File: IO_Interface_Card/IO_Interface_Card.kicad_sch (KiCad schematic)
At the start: 97 parts, among them P1 Conn_02x40_Odd_Even, P2 Conn_02x36_Top_Bottom

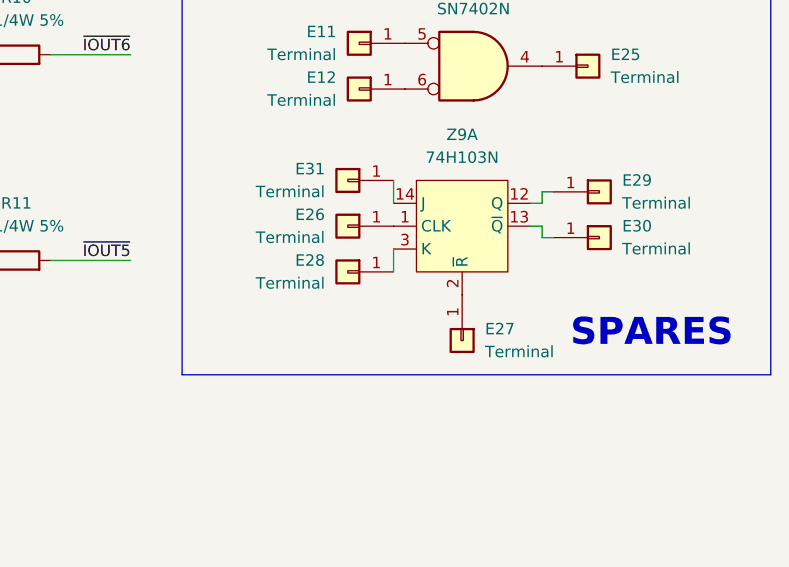
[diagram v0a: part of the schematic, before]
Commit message: Finished Adding Every Chip and Net label in AU1
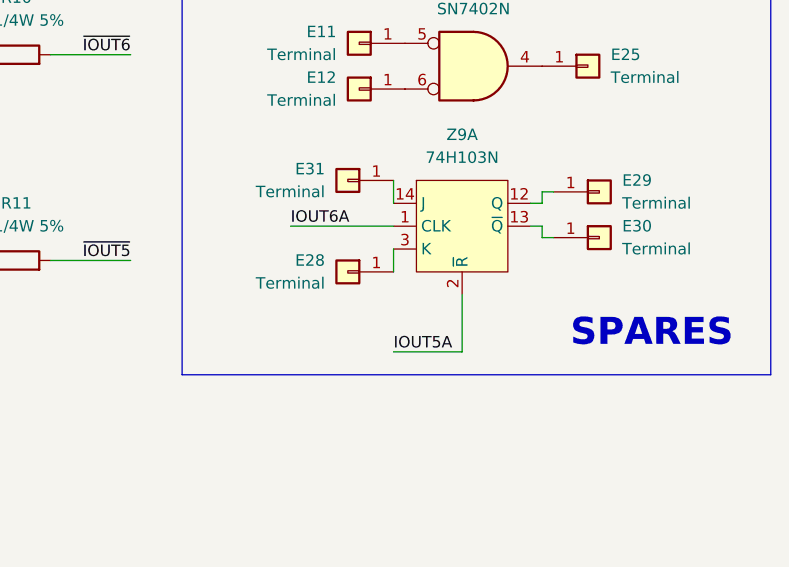
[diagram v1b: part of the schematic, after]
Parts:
- removed E26, E27: Terminal, Connector_PinHeader_2.54mm:PinHeader_1x01_P2.54mm_Horizontal, symbol Connector_Generic:Conn_01x01
- E1, E10, E11, E12, E13, E14, E15, E16, E17, E18, E19, E2, E20, E21, E22, E23, E24, E25, E26, E27, E28, E29, E3, E30, E31, E32, E33, E34, E35, E36, E37, E38, E39, E4, E40, E41, E42, E43, E44, E45, E46, E47, E5, E6, E7, E8, E9: footprint Connector_PinHeader_2.54mm:PinHeader_1x01_P2.54mm_Horizontal -> Connector_PinHeader_2.54mm:PinHeader_1x01_P2.54mm_Vertical
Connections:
- net IOUT5A: now also Z9.2 (~{R})
- net IOUT6A: now also Z9.1 (CLK)
